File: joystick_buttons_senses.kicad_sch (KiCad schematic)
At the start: 73 parts, among them J3 Joystick, J8 DM3AT-SF-PEJM5, Q1 2N2907, Q2 2N2907, SW1 A, SW2 B, SW3 X, SW4 Y, SW5 L, SW6 R, U10 TC1046, U5 24CSM01, U6 23K256, U7 74HC4051, U8 MMA8452Q, U9 AT25DF641A

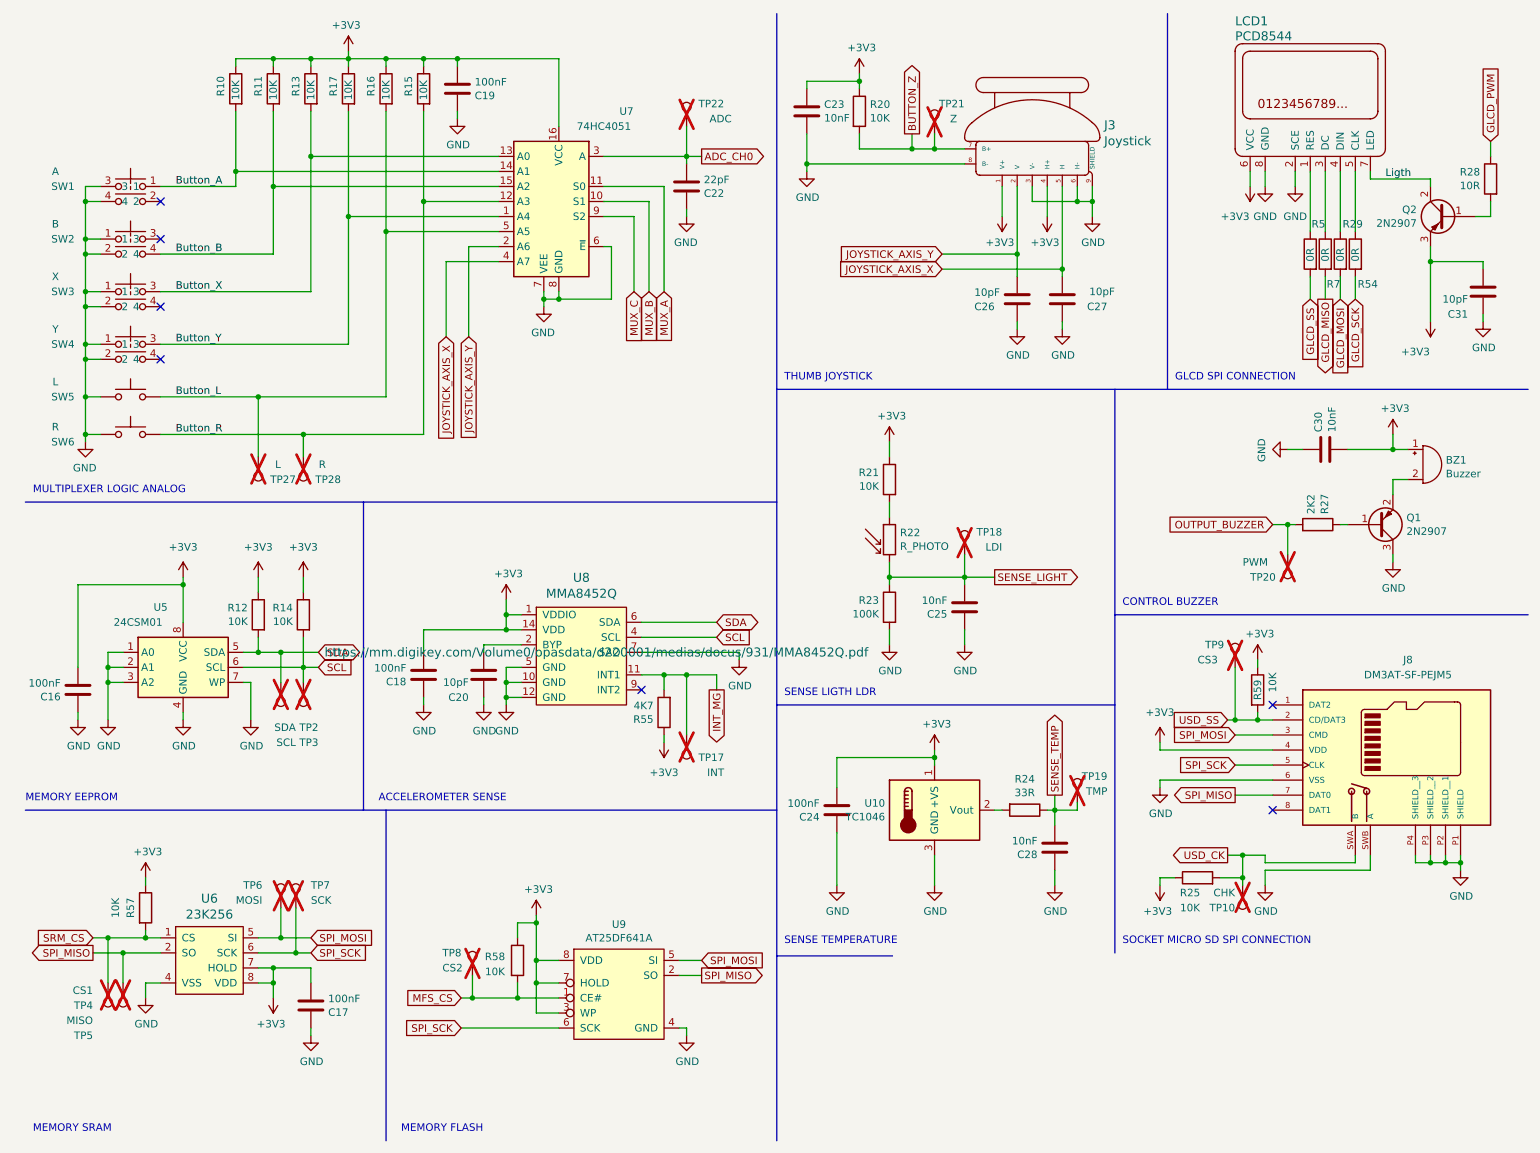
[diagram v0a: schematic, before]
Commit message: 03/12/26/Update BOM & Models VRML
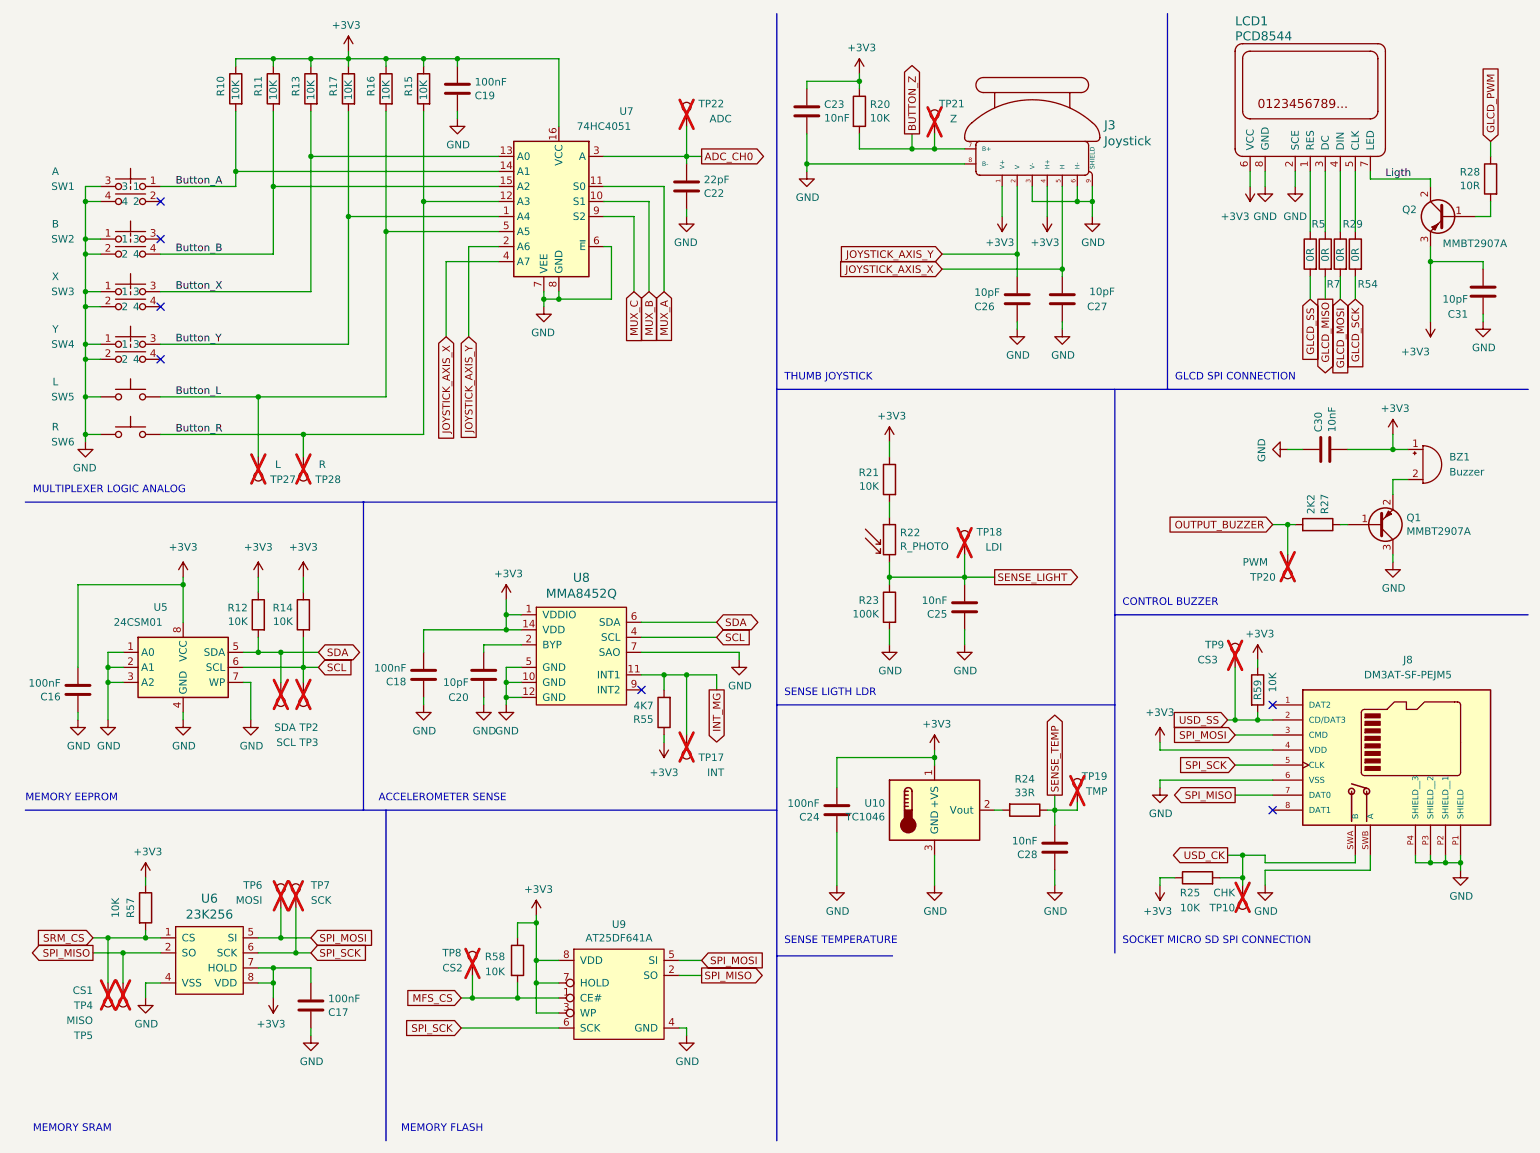
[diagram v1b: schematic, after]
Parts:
- BZ1: footprint Buzzer_Beeper:Buzzer_12x9.5RM7.6 -> x_Buzzer:AT_1224_TWT_5V_2_R; Digikey (none) -> AI-1223-TWT-3V-2-R
- LCD1: Digikey (none) -> SSW-108-01-F-S
- Q1, Q2: value 2N2907 -> MMBT2907A; Digikey (none) -> MMBT2907A-7-F
- R22: Digikey (none) -> N5AC501085
- SW1, SW2, SW3, SW4: Digikey (none) -> TL3300AF160Q
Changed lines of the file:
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@@
 			)
 		)
-		(property "Datasheet" "~"
+		(property "Datasheet" "https://www.farnell.com/datasheets/1580320.pdf"
 			(at 158.75 102.87 0)
 			(effects
@@
 			)
 		)
-		(property "Description" ""
+		(property "Description" "CDS PHOTORESISTOR 100KOHM TO-18"
+			(at 158.75 101.6 0)
+			(effects
+				(font
+					(size 1.27 1.27)
+				)
+				(hide yes)
+			)
+		)
+		(property "Digikey" "N5AC501085"
 			(at 158.75 101.6 0)
 			(effects
@@
 	)
 	(symbol
-		(lib_id "Device:Buzzer")
-		(at 248.92 88.9 0)
-		(unit 1)
-		(exclude_from_sim no)
-		(in_bom yes)
-		(on_board yes)
-		(dnp no)
-		(property "Reference" "BZ1"
-			(at 252.7808 88.1634 0)
-			(effects
-				(font
-					(size 1.27 1.27)
-				)
-				(justify left)
-			)
-		)
-		(property "Value" "Buzzer"
-			(at 252.7808 90.4748 0)
-			(effects
-				(font
-					(size 1.27 1.27)
-				)
-				(justify left)
-			)
-		)
-		(property "Footprint" "Buzzer_Beeper:Buzzer_12x9.5RM7.6"
-			(at 248.285 86.36 90)
-			(effects
-				(font
-					(size 1.27 1.27)
-				)
-				(hide yes)
-			)
-		)
-		(property "Datasheet" "~"
-			(at 248.285 86.36 90)
-			(effects
-				(font
-					(size 1.27 1.27)
-				)
-				(hide yes)
-			)
-		)
-		(property "Description" ""
-			(at 248.92 88.9 0)
-			(effects
-				(font
-					(size 1.27 1.27)
-				)
-				(hide yes)
-			)
-		)
-		(pin "1"
-		)
-		(pin "2"
-		)
-		(instances
-			(project "Game_Cat_R4"
-				(path "/96315415-cfed-47d2-b3dd-d782358bd0df/00000000-0000-0000-0000-00005ce8b424"
-					(reference "BZ1")
-					(unit 1)
-				)
-			)
-		)
-	)
-	(symbol
 		(lib_id "Device:Q_PNP_BEC")
 		(at 241.3 99.06 0)
@@
 			)
 		)
-		(property "Value" "2N2907"
+		(property "Value" "MMBT2907A"
 			(at 246.126 100.203 0)
 			(effects
@@
 			)
 		)
-		(property "Datasheet" "~"
+		(property "Datasheet" "https://mm.digikey.com/Volume0/opasdata/d220001/medias/docus/900/MMBT2907A_Rev2016.pdf"
 			(at 241.3 99.06 0)
 			(effects
@@
 			)
 		)
+		(property "Digikey" "MMBT2907A-7-F"
+			(at 241.3 99.06 0)
+			(effects
+				(font
+					(size 1.27 1.27)
+				)
+				(hide yes)
+			)
+		)
 		(pin "1"
 		)
@@
 			)
 		)
-		(property "Value" "2N2907"
-			(at 247.8786 48.133 0)
+		(property "Value" "MMBT2907A"
+			(at 263.144 51.562 0)
 			(effects
 				(font
@@
 			)
 		)
-		(property "Datasheet" "~"
+		(property "Datasheet" "https://mm.digikey.com/Volume0/opasdata/d220001/medias/docus/900/MMBT2907A_Rev2016.pdf"
 			(at 252.73 46.99 0)
 			(effects
@@
 			)
 		)
+		(property "Digikey" "MMBT2907A-7-F"
+			(at 252.73 46.99 0)
+			(effects
+				(font
+					(size 1.27 1.27)
+				)
+				(hide yes)
+			)
+		)
 		(pin "1"
 		)
@@
 			)
 		)
-		(property "Datasheet" ""
+		(property "Datasheet" "https://mm.digikey.com/Volume0/opasdata/d220001/medias/docus/6129/ssw-1xx-xx-xxx-x-xx-xxx-xx-mkt.pdf"
 			(at 229.87 25.4 0)
 			(effects
@@
 					(size 3.048 3.048)
 				)
+				(hide yes)
+			)
+		)
+		(property "Description" "CONN RCPT 8POS 0.1 GOLD PCB"
+			(at 229.87 25.4 0)
+			(effects
+				(font
+					(size 1.27 1.27)
+				)
+				(hide yes)
 			)
 		)
-		(property "Description" ""
+		(property "Digikey" "SSW-108-01-F-S"
 			(at 229.87 25.4 0)
 			(effects
@@
 					(size 1.524 1.524)
 				)
+				(hide yes)
 			)
 		)
@@
 			)
 		)
-		(property "Datasheet" ""
+		(property "Datasheet" "https://configured-product-images.s3.amazonaws.com/Datasheets/TL3300.pdf"
 			(at 30.48 43.18 0)
 			(effects
@@
 					(size 1.524 1.524)
 				)
+				(hide yes)
 			)
 		)
@@
 			)
 		)
+		(property "Digikey" "TL3300AF160Q"
+			(at 30.48 41.91 0)
+			(effects
+				(font
+					(size 1.27 1.27)
+				)
+				(hide yes)
+			)
+		)
 		(pin "1"
 		)
@@
 			)
 		)
-		(property "Datasheet" ""
+		(property "Datasheet" "https://configured-product-images.s3.amazonaws.com/Datasheets/TL3300.pdf"
 			(at 30.48 52.07 0)
 			(effects
@@
 					(size 1.524 1.524)
 				)
+				(hide yes)
 			)
 		)
@@
 			)
 		)
+		(property "Digikey" "TL3300AF160Q"
+			(at 30.48 50.8 0)
+			(effects
+				(font
+					(size 1.27 1.27)
+				)
+				(hide yes)
+			)
+		)
 		(pin "1"
 		)
@@
 			)
 		)
-		(property "Datasheet" ""
+		(property "Datasheet" "https://configured-product-images.s3.amazonaws.com/Datasheets/TL3300.pdf"
 			(at 30.48 60.96 0)
 			(effects
@@
 					(size 1.524 1.524)
 				)
+				(hide yes)
 			)
 		)
@@
 			)
 		)
+		(property "Digikey" "TL3300AF160Q"
+			(at 30.48 59.69 0)
+			(effects
+				(font
+					(size 1.27 1.27)
+				)
+				(hide yes)
+			)
+		)
 		(pin "1"
 		)
@@
 			)
 		)
-		(property "Datasheet" ""
+		(property "Datasheet" "https://configured-product-images.s3.amazonaws.com/Datasheets/TL3300.pdf"
 			(at 30.48 69.85 0)
 			(effects
@@
 					(size 1.524 1.524)
 				)
+				(hide yes)
 			)
 		)
@@
 			)
 		)
+		(property "Digikey" "TL3300AF160Q"
+			(at 30.48 68.58 0)
+			(effects
+				(font
+					(size 1.27 1.27)
+				)
+				(hide yes)
+			)
+		)
 		(pin "1"
 		)
@@
 					(unit 1)
 				)
+			)
+		)
+	)
+	(symbol
+		(lib_id "Device:Buzzer")
+		(at 248.92 88.9 0)
+		(unit 1)
+		(exclude_from_sim no)
+		(in_bom yes)
+		(on_board yes)
+		(dnp no)
+		(fields_autoplaced yes)
+		(property "Reference" "BZ1"
+			(at 253.365 87.63 0)
+			(effects
+				(font
+					(size 1.27 1.27)
+				)
+				(justify left)
+			)
+		)
+		(property "Value" "Buzzer"
+			(at 253.365 90.17 0)
+			(effects
+				(font
+					(size 1.27 1.27)
+				)
+				(justify left)
+			)
+		)
+		(property "Footprint" "x_Buzzer:AT_1224_TWT_5V_2_R"
+			(at 248.285 86.36 90)
+			(effects
+				(font
+					(size 1.27 1.27)
+				)
+				(hide yes)
+			)
+		)
+		(property "Datasheet" "https://puiaudio.com/file/specs-AI-1223-TWT-3V-2-R.pdf"
+			(at 248.285 86.36 90)
+			(effects
+				(font
+					(size 1.27 1.27)
+				)
+				(hide yes)
+			)
+		)
+		(property "Description" "BUZZER MAGNETIC 3V 12MM TH"
+			(at 248.92 88.9 0)
+			(effects
+				(font
+					(size 1.27 1.27)
+				)
+				(hide yes)
+			)
+		)
+		(property "Digikey" "AI-1223-TWT-3V-2-R"
+			(at 248.92 88.9 0)
+			(effects
+				(font
+					(size 1.27 1.27)
+				)
+				(hide yes)
+			)
+		)
+		(pin "1"
+		)
+		(pin "2"
+		)
+		(instances
+			(project "Game_Cat_R4"
+				(path "/96315415-cfed-47d2-b3dd-d782358bd0df/00000000-0000-0000-0000-00005ce8b424"
+					(reference "BZ1")
+					(unit 1)
+				)
